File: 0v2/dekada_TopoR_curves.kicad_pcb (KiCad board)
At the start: 2 copper layers, 49.8 x 33 mm, 43 parts, among them P1 CONN_02X10, P2 CONN_02X10, P3 CONN_02X10, P4 CONN_02X10, P5 CONN_01X02, P6 CONN_01X02, P7 CONN_01X02

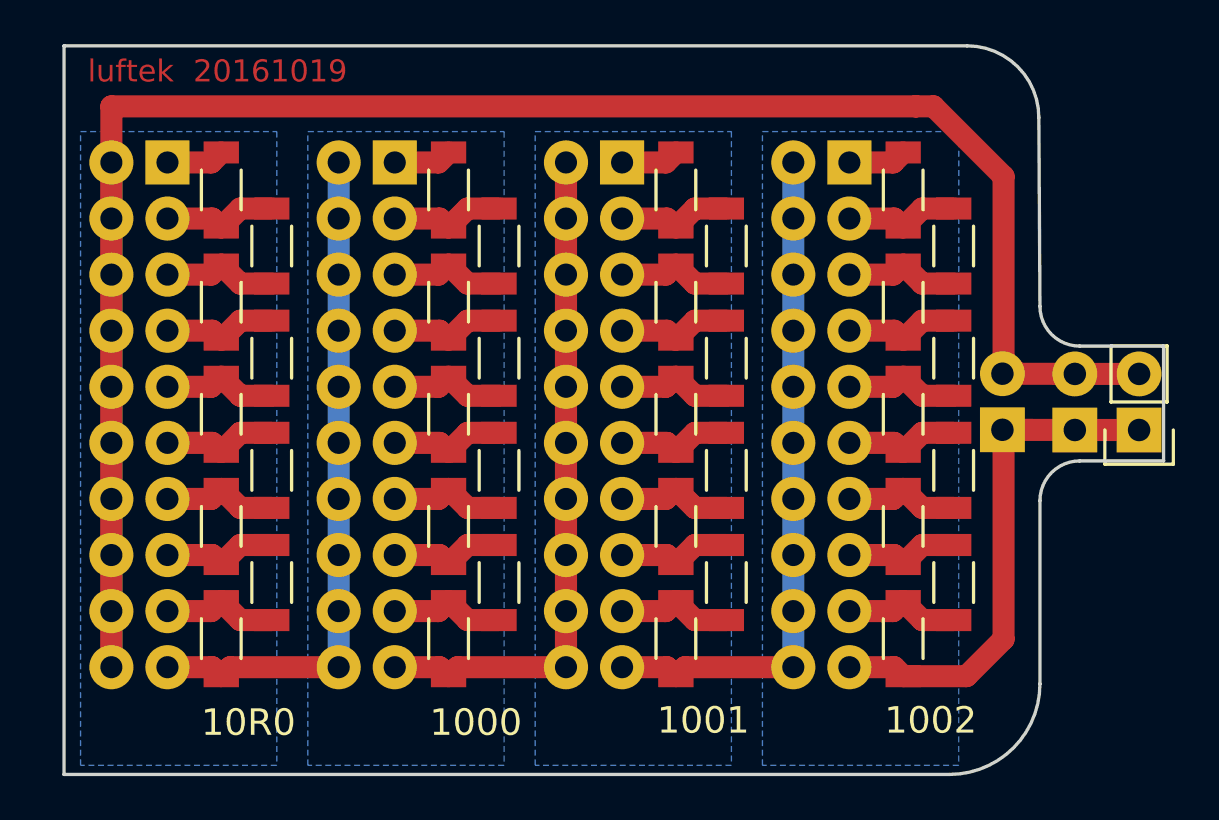
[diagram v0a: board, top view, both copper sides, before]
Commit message: Version 0v3
assembled, tested, working
no downsides or need for improvement found for now
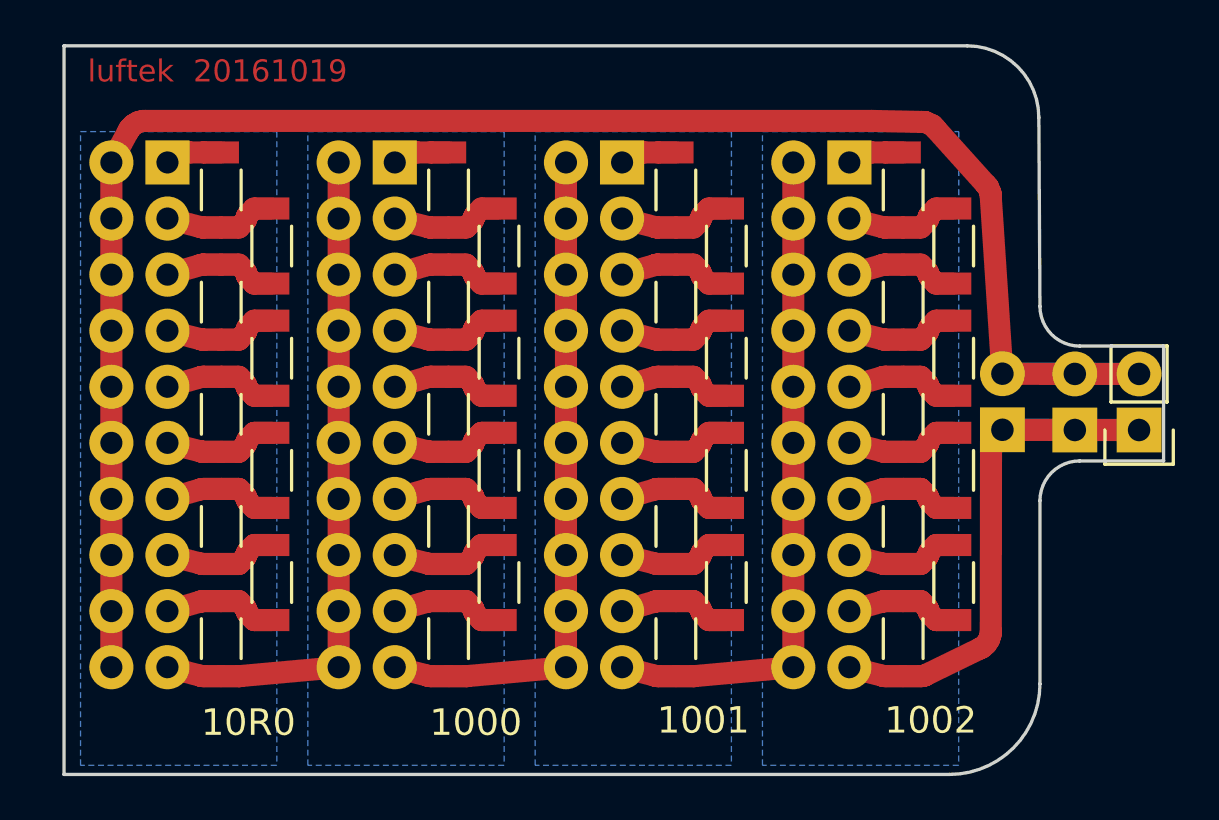
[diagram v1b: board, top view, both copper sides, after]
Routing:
- net Net-(P2-Pad19): track 53.8 -> 30.7 mm
- net Net-(P1-Pad10): track 105.4 -> 85.7 mm
- net Net-(P4-Pad19): track 23.8 -> 28.9 mm
